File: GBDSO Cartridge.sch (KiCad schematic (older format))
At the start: 75 parts, among them J1 MJ-3523-SMT-TR, J2 MJ-3523-SMT-TR, J3 EdgeConnector, J5 Conn_01x02, J6 Conn_01x02, P1 100k, P2 100k, SW1 SW_SPDT, SW2 SW_SPDT, U1 TL072, U2 DS1267_SOIC, U3 TL072, U4 MAX114CAG, U5 74HC175D, U6 74HC138D, U7 AT27C256R, U8 TLC272, U9 MAX828

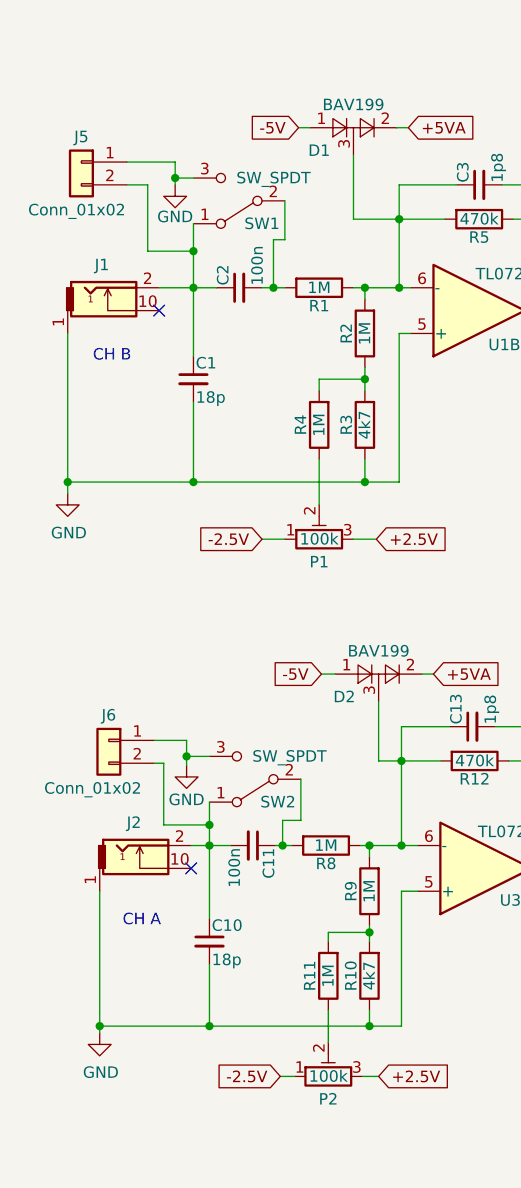
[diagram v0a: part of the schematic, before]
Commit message: big v2 update, hopefully everything is ok now
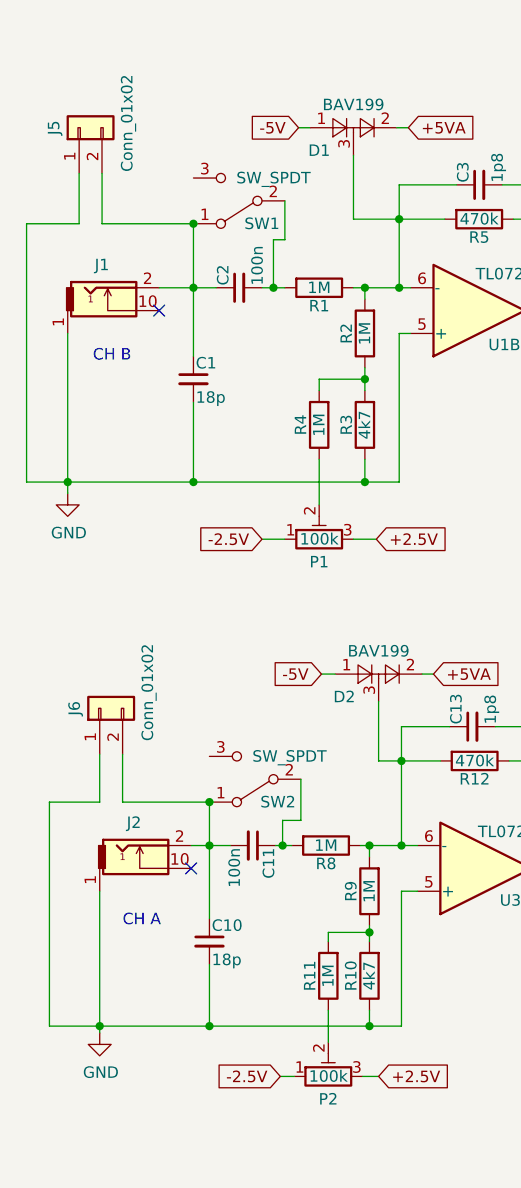
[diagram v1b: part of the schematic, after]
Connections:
- net GND: no longer SW1.3 (C), SW2.3 (C)
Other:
- moved on the sheet: J5, J6
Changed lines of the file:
@@
 Connection ~ 870  4900
-Wire Wire Line
-	1350 3920 1350 4020
 Wire Wire Line
 	1750 3820 1750 4000
@@
 L Connector_Generic:Conn_01x02 J5
 U 1 1 5CB7D891
-P 790 1120
-F 0 "J5" H 790 1230 50  0000 C CNN
-F 1 "Conn_01x02" H 810 910 50  0000 C CNN
-F 2 "Connector_PinHeader_2.54mm:PinHeader_1x02_P2.54mm_Horizontal" H 790 1120 50  0001 C CNN
-F 3 "~" H 790 1120 50  0001 C CNN
-	1    790  1120
-	-1   0    0    -1
+P 780 970
+F 0 "J5" H 780 1080 50  0000 C CNN
+F 1 "Conn_01x02" H 800 760 50  0000 C CNN
+F 2 "Connector_PinHeader_2.54mm:PinHeader_1x02_P2.54mm_Horizontal" H 780 970 50  0001 C CNN
+F 3 "~" H 780 970 50  0001 C CNN
+	1    780  970
+	0    -1   -1   0
 $EndComp
 $Comp
 L Connector_Generic:Conn_01x02 J6
 U 1 1 5CB7E2B7
-P 910 3650
-F 0 "J6" H 910 3760 50  0000 C CNN
-F 1 "Conn_01x02" H 980 3440 50  0000 C CNN
-F 2 "Connector_PinHeader_2.54mm:PinHeader_1x02_P2.54mm_Horizontal" H 910 3650 50  0001 C CNN
-F 3 "~" H 910 3650 50  0001 C CNN
-	1    910  3650
-	-1   0    0    -1
-$EndComp
-$Comp
-L power:GND #PWR0127
-U 1 1 5CBDB355
-P 1250 3760
-F 0 "#PWR0127" H 1250 3510 50  0001 C CNN
-F 1 "GND" H 1250 3610 50  0000 C CNN
-F 2 "" H 1250 3760 50  0001 C CNN
-F 3 "" H 1250 3760 50  0001 C CNN
-	1    1250 3760
-	1    0    0    -1
-$EndComp
-Wire Wire Line
-	1080 1220 1080 1510
-$Comp
-L power:GND #PWR0128
-U 1 1 5CCF1BAC
-P 1200 1220
-F 0 "#PWR0128" H 1200 970 50  0001 C CNN
-F 1 "GND" H 1200 1080 50  0000 C CNN
-F 2 "" H 1200 1220 50  0001 C CNN
-F 3 "" H 1200 1220 50  0001 C CNN
-	1    1200 1220
-	1    0    0    -1
+P 870 3510
+F 0 "J6" H 870 3620 50  0000 C CNN
+F 1 "Conn_01x02" H 940 3300 50  0000 C CNN
+F 2 "Connector_PinHeader_2.54mm:PinHeader_1x02_P2.54mm_Horizontal" H 870 3510 50  0001 C CNN
+F 3 "~" H 870 3510 50  0001 C CNN
+	1    870  3510
+	0    -1   -1   0
 $EndComp
 Text Notes 840  2000 0    50   ~ 0
@@
 Wire Wire Line
 	8090 5010 8350 5010
-Wire Wire Line
-	1200 1220 1200 1190
-Wire Wire Line
-	1200 1190 1280 1190
-Wire Wire Line
-	1080 1220 990  1220
-Wire Wire Line
-	1200 1120 1200 1190
-Wire Wire Line
-	990  1120 1200 1120
-Connection ~ 1200 1190
-Wire Wire Line
-	1080 1510 1280 1510
-Wire Wire Line
-	1280 1390 1280 1510
-Connection ~ 1280 1510
-Wire Wire Line
-	1280 1510 1280 1670
-Wire Wire Line
-	1350 4020 1150 4020
-Wire Wire Line
-	1150 4020 1150 3750
-Wire Wire Line
-	1150 3750 1110 3750
-Connection ~ 1350 4020
-Wire Wire Line
-	1350 4020 1350 4110
-Wire Wire Line
-	1110 3650 1250 3650
-Wire Wire Line
-	1250 3650 1250 3720
-Connection ~ 1250 3720
-Wire Wire Line
-	1250 3720 1250 3760
-Wire Wire Line
-	1250 3720 1350 3720
 Text GLabel 10550 2840 1    50   Input ~ 0
 +5V
@@
 	-1   0    0    1
 $EndComp
+Wire Wire Line
+	1350 3920 1350 4110
+Wire Wire Line
+	1280 1390 1280 1670
+Wire Wire Line
+	780  1170 780  1390
+Wire Wire Line
+	780  1390 550  1390
+Wire Wire Line
+	550  1390 550  2520
+Wire Wire Line
+	550  2520 730  2520
+Wire Wire Line
+	880  1170 880  1390
+Wire Wire Line
+	880  1390 1280 1390
+Connection ~ 1280 1390
+Wire Wire Line
+	970  3710 970  3920
+Wire Wire Line
+	970  3920 1350 3920
+Connection ~ 1350 3920
+Wire Wire Line
+	870  3710 870  3920
+Wire Wire Line
+	870  3920 650  3920
+Wire Wire Line
+	650  3920 650  4900
+Wire Wire Line
+	650  4900 870  4900
 Wire Bus Line
 	5370 2545 5370 3350
